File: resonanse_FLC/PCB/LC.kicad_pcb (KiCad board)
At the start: 2 copper layers, 93 x 25 mm, 39 parts, among them J1 Conn_01x02, J2 Conn_01x02, J3 Conn_01x02, J4 Conn_01x02, J5 RF, Q1 BFT92, Q2 BFT92, Q3 BC857, Q4 BF998, Q5 SS9018, U1 L78L05_TO92

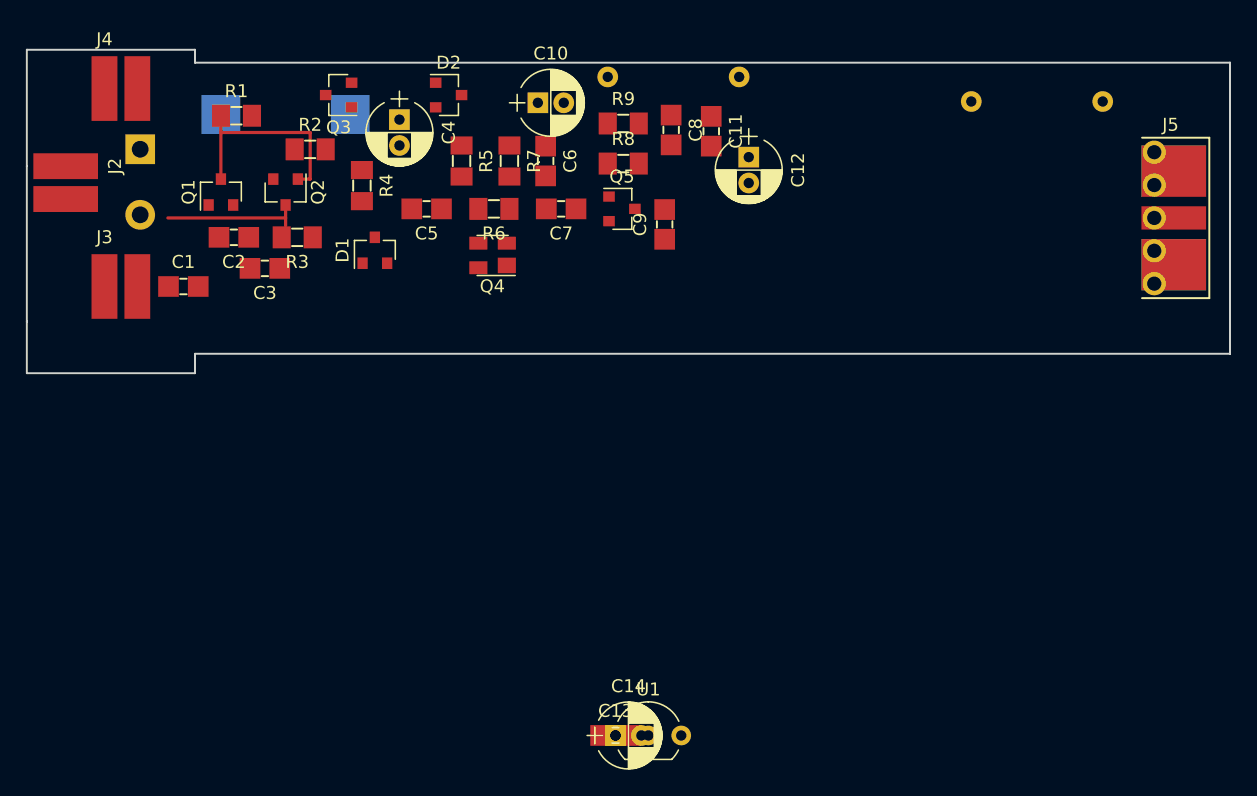
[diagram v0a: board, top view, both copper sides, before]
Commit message: finish PCB
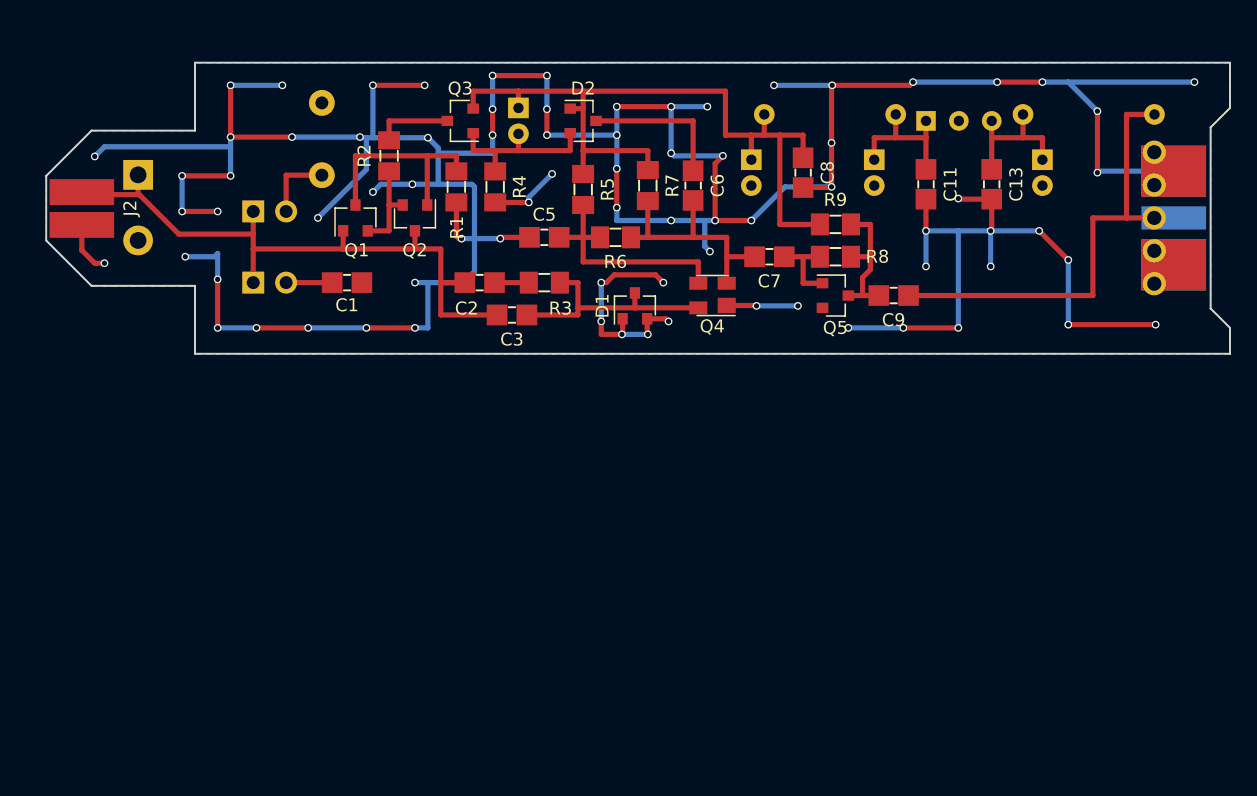
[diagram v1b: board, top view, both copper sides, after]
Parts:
- C10, C12, C14, C4, J5, U1: moved to B.Cu
- J3, J4: footprint lc_probe:SolderWirePad_double_SMD_2x5mm -> Pin_Headers:Pin_Header_Straight_1x02_Pitch2.54mm; moved to B.Cu
- L1: footprint lc_probe:Choke_Toroid_horizontal_Diameter10-5mm_Amidon-T37_2 -> Choke_Toroid_ThroughHole:Choke_Toroid_6,5x13mm_Vertical
- moved C14 55.4 mm to (181.5, 60.5), turned to 270 degrees
- moved U1 53.2 mm to (172.5, 57.5)
- moved C13 51.6 mm to (177.6, 62.4), turned to 270 degrees
- moved D1 20.6 mm to (150.0, 71.8)
- moved C3 19.4 mm to (140.5, 72.5)
- moved R3 19.4 mm to (143.0, 70.0)
- moved C2 19.3 mm to (138.0, 70.0)
- moved C9 18.5 mm to (170.0, 71.0), turned to 180 degrees
- moved R9 18.2 mm to (165.5, 65.5)
- moved R8 17.9 mm to (165.5, 68.0)
- moved R1 17.9 mm to (136.2, 62.6), turned to 270 degrees
- moved Q5 17.8 mm to (165.5, 71.0)
- moved Q4 17.3 mm to (156.0, 71.0)
- moved C11 17.1 mm to (172.5, 62.4)
- moved C10 17.1 mm to (159.0, 60.5), turned to 270 degrees
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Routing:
- net GND: track 0.00 -> 337.2 mm, vias 0 -> 77
- net Net-(C10-Pad1): track 0.00 -> 60.7 mm
- net Net-(C2-Pad2): track 10.7 -> 50.2 mm
- net Net-(C9-Pad1): track 0.00 -> 35.2 mm
- net Net-(C6-Pad2): track 0.00 -> 18.8 mm
- net Net-(C3-Pad1): track 0.00 -> 18.3 mm
- net Net-(C5-Pad1): track 0.00 -> 18.1 mm
- net Net-(C4-Pad2): track 0.00 -> 13.1 mm
- net Net-(C6-Pad1): track 0.00 -> 11.4 mm
- net Net-(C11-Pad1): track 0.00 -> 11.2 mm
- net Net-(C13-Pad1): track 0.00 -> 11.2 mm
- net Net-(C9-Pad2): track 0.00 -> 11.1 mm
- net Net-(Q1-Pad2): track 0.00 -> 7.30 mm
- net Net-(C7-Pad1): track 0.00 -> 6.30 mm
- net Net-(Q3-Pad3): track 0.00 -> 6.00 mm
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- added copper zone on B.Cu, net GND
- added copper zone on F.Cu, net GND
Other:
- board size 93 x 25 mm -> 91.5 x 22.5 mm
- net class Default: trace_width 0.25 -> 0.4
